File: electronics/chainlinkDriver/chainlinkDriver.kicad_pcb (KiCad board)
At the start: 2 copper layers, 198.1 x 30.5 mm, 65 parts, among them J10 Sensor, J11 Sensor, J12 Motor, J13 Motor, J14 Sensor, J15 Sensor, J16 Power, J17 Power, J18 Power, J19 IDC, J20 IDC, J3 Motor, J5 Motor, J6 Motor, J7 Motor, J8 Sensor, J9 Sensor, U1 74HC595, U10 TPL7407L, U2 TPL7407L, U3 74HC125, U4 74HC165, U5 74HC595, U6 TPL7407L, U7 74HC595, U8 TPL7407L, U9 74HC595

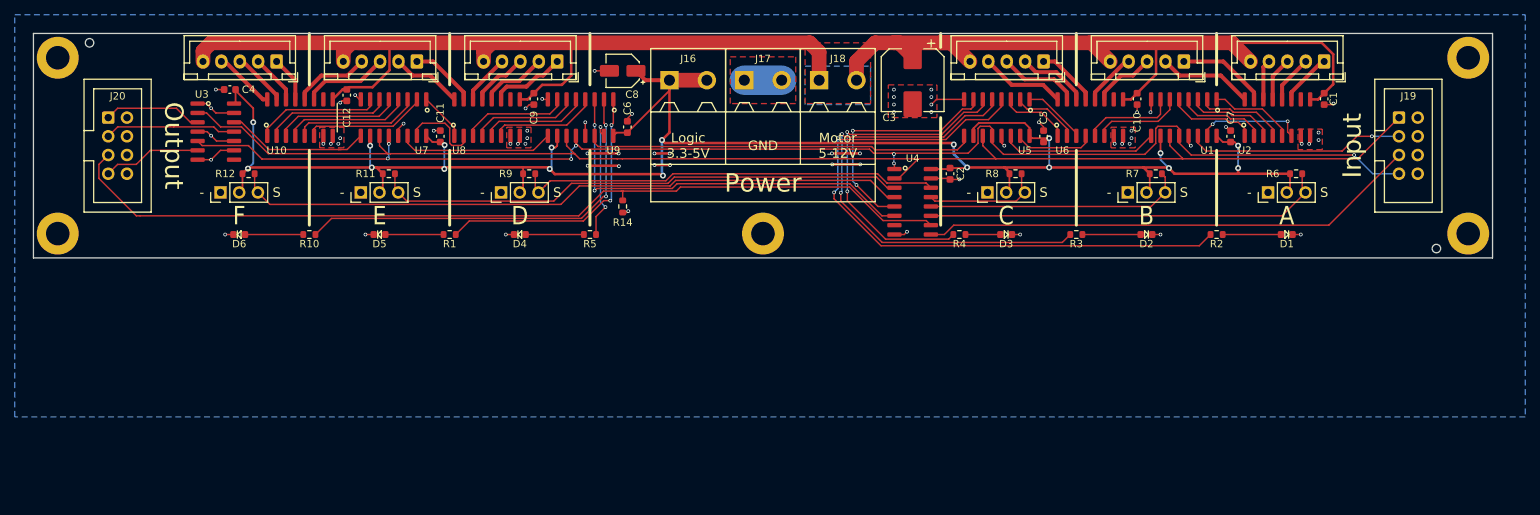
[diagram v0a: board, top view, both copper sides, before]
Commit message: Add Chainlink KiCad schematics and libs
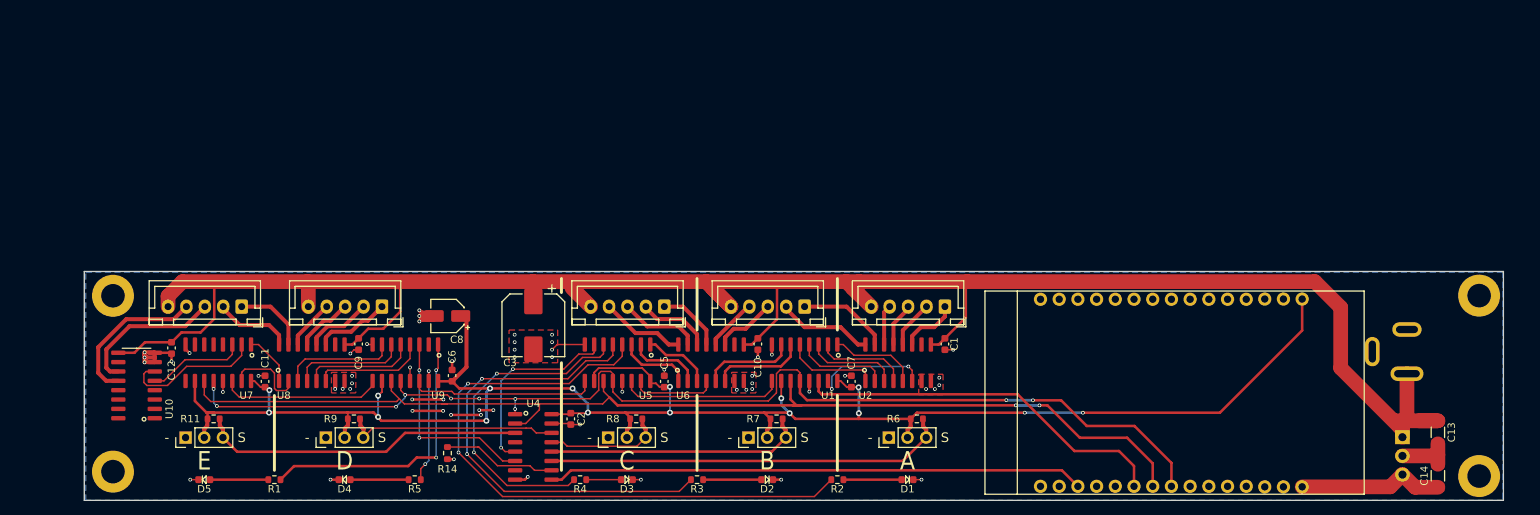
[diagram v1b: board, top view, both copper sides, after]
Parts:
- removed C4: 0.1uF, Capacitor_SMD:C_0603_1608Metric
- removed D6: LED, ModifiedSymbols:LED_0603_1608Metric_Silkscreen
- removed H5: MountingHole, MountingHole:MountingHole_3.2mm_M3_ISO7380_Pad
- removed H6, H7: MountingHole, JLCPCB:AssemblyToolingHole
- removed J13: Motor, Connector_JST:JST_XH_B5B-XH-A_1x05_P2.50mm_Vertical
- removed J15: Sensor, Connector_PinHeader_2.54mm:PinHeader_1x03_P2.54mm_Vertical
- removed J16, J17, J18: Power, ScrewTerminals:Generic-5.08-2P
- removed J19, J20: IDC, ModifiedSymbols:IDC-Header_2x04_P2.54mm_Vertical
- removed R10: 220R, Resistor_SMD:R_0603_1608Metric
- removed R12: 47k, Resistor_SMD:R_0603_1608Metric
- added C13: 10uF, Capacitor_SMD:C_1206_3216Metric_Pad1.33x1.80mm_HandSolder, F.Cu at (216.1, 79.6)
- added C14: 22uF, Capacitor_SMD:C_1206_3216Metric_Pad1.33x1.80mm_HandSolder, F.Cu at (216.1, 85.5)
- added J1: Barrel_Jack_Switch, Library:PJ202, F.Cu at (217.4, 74.3)
- added U11: MyESP32, Library:MyESP32, F.Cu at (208.0, 91.0)
- U3: value 74HC125 -> LM7805_TO220; footprint ModifiedSymbols:SOIC-14_3.9x8.7mm_P1.27mm_silk -> Library:TO-220-3_Vertical
- moved U3 161.2 mm to (207.2, 75.0), turned to -90 degrees
- moved J5 61.3 mm to (130.1, 62.5)
- moved U1 61.3 mm to (130.1, 70.1)
- moved C1 61.3 mm to (149.2, 67.6)
- moved C2 61.3 mm to (98.4, 77.7)
- moved C5 61.3 mm to (111.1, 72.7)
- moved C7 61.3 mm to (136.5, 72.7)
- moved J10 61.3 mm to (103.4, 80.3)
- moved J8 61.3 mm to (141.5, 80.3)
- moved J9 61.3 mm to (122.5, 80.3)
- moved R7 61.3 mm to (126.3, 77.7)
- moved U4 61.3 mm to (93.3, 81.5)
- moved U5 61.3 mm to (104.7, 70.1)
- moved C3 61.3 mm to (93.3, 65.0)
- moved D1 61.3 mm to (144.1, 86.0)
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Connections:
- C11 pad 1: +3V3 -> +3.3V
- C2 pad 1: +3V3 -> +3.3V
- C5 pad 1: +3V3 -> +3.3V
- C6 pad 1: +3V3 -> +3.3V
- C7 pad 1: +3V3 -> +3.3V
- C8 pad 1: +3V3 -> +3.3V
- H1 pad 1: (no net) -> unconnected-(H1-Pad1)
- H2 pad 1: (no net) -> unconnected-(H2-Pad1)
- H3 pad 1: (no net) -> unconnected-(H3-Pad1)
- H4 pad 1: (no net) -> unconnected-(H4-Pad1)
- J10 pad 2: +3V3 -> +3.3V
- J11 pad 2: +3V3 -> +3.3V
- J14 pad 2: +3V3 -> +3.3V
- J8 pad 2: +3V3 -> +3.3V
- J9 pad 2: +3V3 -> +3.3V
- R11 pad 1: +3V3 -> +3.3V
- R6 pad 1: +3V3 -> +3.3V
- R7 pad 1: +3V3 -> +3.3V
- R8 pad 1: +3V3 -> +3.3V
- R9 pad 1: +3V3 -> +3.3V
- U1 pad 10: +3V3 -> +3.3V
- U1 pad 11: /CLOCK_IN -> /CLOCK
- U1 pad 12: /LATCH_IN -> /LATCH
- U1 pad 14: /MOTOR_IN -> /MOTOR_DATA
- U1 pad 16: +3V3 -> +3.3V
- U10 pad 1: /MOTOR_F_PHASE_D -> unconnected-(U10-I1-Pad1)
- U10 pad 10: (no net) -> unconnected-(U10-O7-Pad10)
- U10 pad 13: /OUT_F_PHASE_A -> unconnected-(U10-O4-Pad13)
- U10 pad 14: /OUT_F_PHASE_B -> unconnected-(U10-O3-Pad14)
- U10 pad 15: /OUT_F_PHASE_C -> unconnected-(U10-O2-Pad15)
- U10 pad 16: /OUT_F_PHASE_D -> unconnected-(U10-O1-Pad16)
- U10 pad 2: /MOTOR_F_PHASE_C -> unconnected-(U10-I2-Pad2)
- U10 pad 3: /MOTOR_F_PHASE_B -> unconnected-(U10-I3-Pad3)
- U10 pad 4: /MOTOR_F_PHASE_A -> unconnected-(U10-I4-Pad4)
- U2 pad 10: (no net) -> unconnected-(U2-O7-Pad10)
- U3 pad 1: GND -> +12V
- U3 pad 2: /CLOCK_IN -> GND
- U3 pad 3: /CLOCK_OUT -> +5V
- U4 pad 1: /LATCH_IN -> /LATCH
- U4 pad 16: +3V3 -> +3.3V
- U4 pad 2: /CLOCK_IN -> /CLOCK
- U4 pad 4: /SENSOR_F -> unconnected-(U4-F-Pad4)
- U4 pad 7: (no net) -> unconnected-(U4-~{QH}-Pad7)
- U4 pad 9: /SENSOR_OUT -> /SENSOR_DATA
- U5 pad 10: +3V3 -> +3.3V
- U5 pad 11: /CLOCK_IN -> /CLOCK
- U5 pad 12: /LATCH_IN -> /LATCH
- U5 pad 16: +3V3 -> +3.3V
- U6 pad 10: (no net) -> unconnected-(U6-O7-Pad10)
- U7 pad 10: +3V3 -> +3.3V
- U7 pad 11: /CLOCK_IN -> /CLOCK
- U7 pad 12: /LATCH_IN -> /LATCH
- U7 pad 16: +3V3 -> +3.3V
- U7 pad 4: /MOTOR_F_PHASE_A -> unconnected-(U7-QE-Pad4)
- U7 pad 5: /MOTOR_F_PHASE_B -> unconnected-(U7-QF-Pad5)
- U7 pad 6: /MOTOR_F_PHASE_C -> unconnected-(U7-QG-Pad6)
- U7 pad 7: /MOTOR_F_PHASE_D -> unconnected-(U7-QH-Pad7)
- U8 pad 10: (no net) -> unconnected-(U8-O7-Pad10)
- U9 pad 10: +3V3 -> +3.3V
- U9 pad 11: /CLOCK_IN -> /CLOCK
- U9 pad 12: /LATCH_IN -> /LATCH
- U9 pad 16: +3V3 -> +3.3V
- U9 pad 2: /LED_F -> unconnected-(U9-QC-Pad2)
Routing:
- net +3V3: track 267.1 -> 0.00 mm, vias 18 -> 0
- net +3.3V: track 0.00 -> 255.4 mm, vias 0 -> 16
- net /CLOCK_IN: track 188.1 -> 0.00 mm
- net /LATCH_IN: track 186.0 -> 0.00 mm, vias 7 -> 0
- net /LATCH: track 0.00 -> 158.7 mm, vias 0 -> 10
- net /CLOCK: track 0.00 -> 156.9 mm, vias 0 -> 2
- net /SENSOR_IN: track 123.8 -> 15.6 mm
- net /SENSOR_F: track 92.1 -> 0.00 mm
- net /SENSOR_DATA: track 0.00 -> 72.9 mm
- net /SENSOR_OUT: track 68.0 -> 0.00 mm
- net /LED_F: track 54.9 -> 0.00 mm, vias 2 -> 0
- net /MOTOR_DATA: track 0.00 -> 51.2 mm
- net +12V: track 226.3 -> 277.4 mm
- net /MOTOR_IN: track 29.6 -> 0.00 mm, vias 1 -> 0
- net /LOOPBACK_B: track 55.3 -> 27.0 mm
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- removed copper zone on B.Cu, net +12V
- removed copper zone on F.Cu, net +12V
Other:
- board size 198.1 x 30.5 mm -> 192.7 x 31.1 mm
- net class Default removed
- net class save removed
- board text removed: "DATE: YYYY-MM-DD COMMIT: deadbeef"
- board text removed: "F"
- board text removed: "GND"
- board text removed: "Input"
- board text removed: "Logic 3.3-5V"
- board text removed: "Motor 5-12V"
- board text removed: "Output"
- board text removed: "Power"
- board text removed: "Splitflap Chainlink Driver"
- board text removed: "https://github.com/scottbez1/splitflap"
- board text removed: "v1.1"
